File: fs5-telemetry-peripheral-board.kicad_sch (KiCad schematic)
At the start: 36 parts, among them J1 ATS668LSM, J2 Potentiometer, J3 Conn_01x10_Pin, J4 Strain Gauge, J5 1x8 Tire Surface Temperature 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, J6 Tire Temperature Sensor, J7 1x1 Tire Air Temperature Sens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, J8 Conn_01x09_Pin, J9 Conn_01x04_MountingPin, U1 LM2907M/NOPB, U2 LM7805CV, U3 INA125U, U4 ISO1050DUB

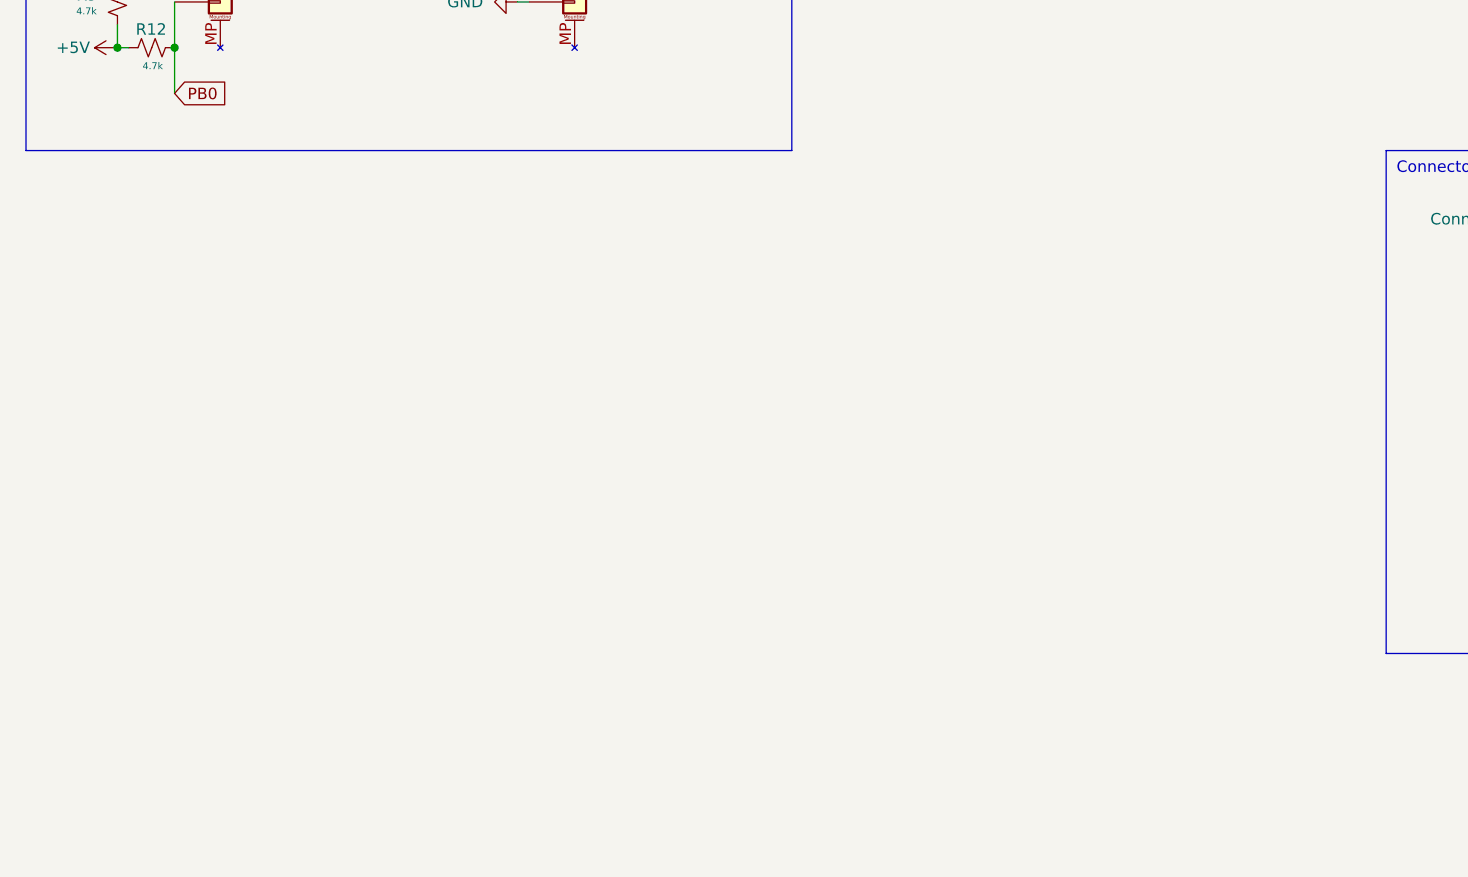
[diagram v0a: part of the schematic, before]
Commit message: added
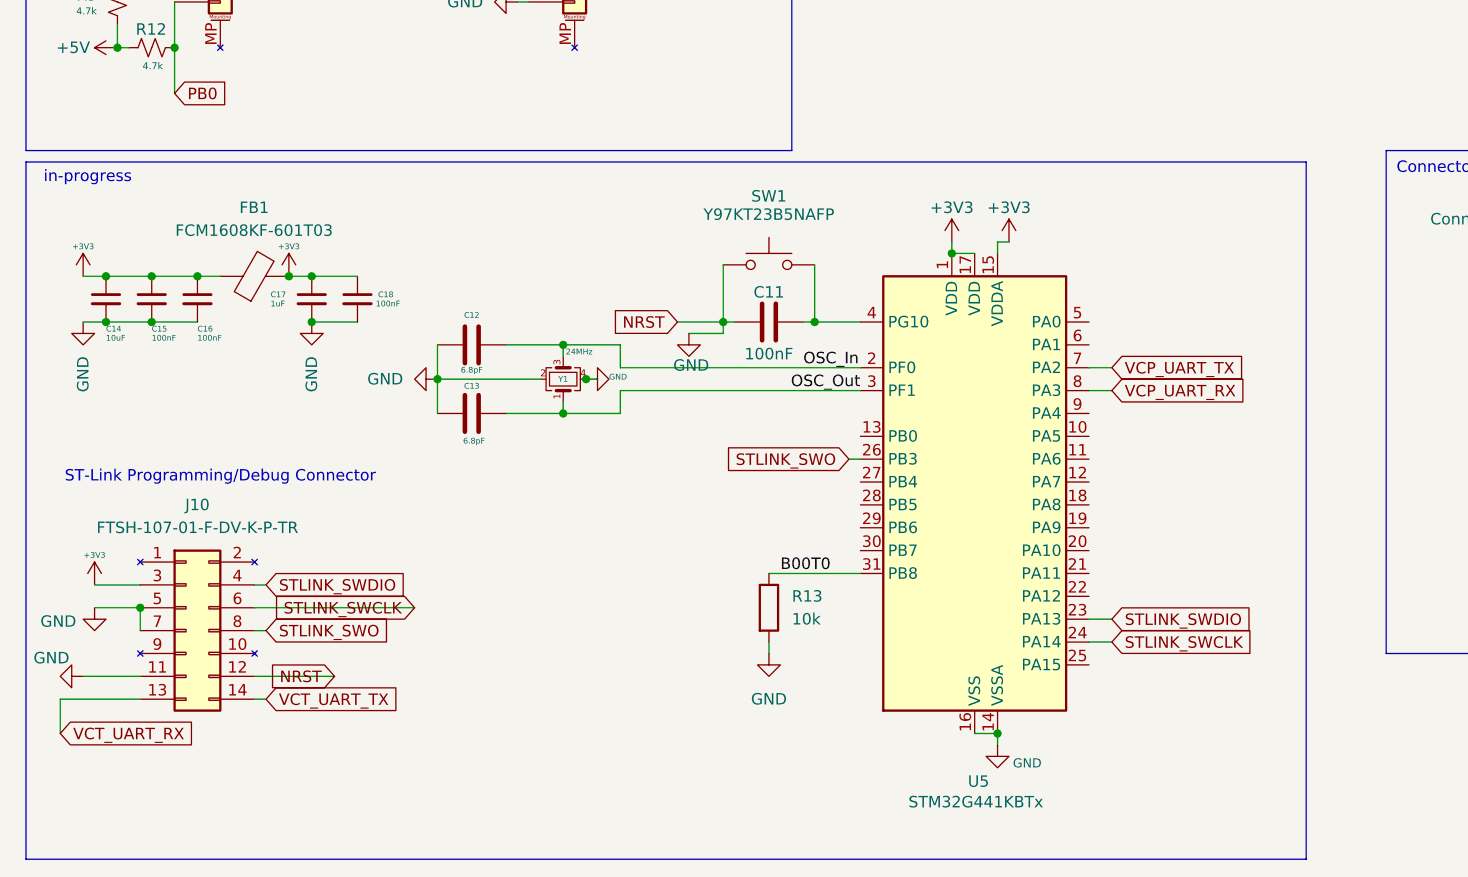
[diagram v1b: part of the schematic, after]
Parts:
- added C11: 100nF, symbol Device:C
- added C12, C13: 6.8pF, symbol Device:C
- added C14: 10uF, symbol Device:C_Small
- added C15, C16, C18: 100nF, symbol Device:C_Small
- added C17: 1uF, symbol Device:C_Small
- added FB1: FCM1608KF-601T03, symbol Device:FerriteBead
- added J10: FTSH-107-01-F-DV-K-P-TR, symbol Connector_Generic:Conn_02x07_Odd_Even
- added R13: 10k, symbol Device:R
- added SW1: Y97KT23B5NAFP, symbol Switch:SW_Push
- added U5: STM32G441KBTx, Package_QFP:LQFP-32_7x7mm_P0.8mm, symbol MCU_ST_STM32G4:STM32G441KBTx
- added Y1: 24MHz, symbol Device:Crystal_GND24_Small
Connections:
- net GND: now also C11.1, C12.1, C13.1, C14.2, C15.2, C16.2, C17.2, C18.2, J10.11 (Pin_11), J10.12 (Pin_12), J10.5 (Pin_5), J10.7 (Pin_7), R13.2, SW1.1, U5.14 (VSSA), U5.16 (VSS), U5.32 (VSS), Y1.2 (G), Y1.4 (G)
- new net: C11.2, SW1.2, U5.4 (PG10)
- new net +3V3: C14.1, C15.1, C16.1, C17.1, C18.1, FB1.1, FB1.2, J10.3 (Pin_3), U5.1 (VDD), U5.15 (VDDA), U5.17 (VDD)
- new net B00T0: R13.1, U5.31 (PB8)
- new net OSC_In: C12.2, U5.2 (PF0), Y1.3
- new net OSC_Out: C13.2, U5.3 (PF1), Y1.1
- new net STLINK_SWCLK: J10.6 (Pin_6), U5.24 (PA14)
- new net STLINK_SWDIO: J10.4 (Pin_4), U5.23 (PA13)
- new net STLINK_SWO: J10.8 (Pin_8), U5.26 (PB3)
- new net VCP_UART_RX: U5.8 (PA3)
- new net VCP_UART_TX: U5.7 (PA2)
- new net VCT_UART_RX: J10.13 (Pin_13)
- new net VCT_UART_TX: J10.14 (Pin_14)
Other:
- note added: "ST-Link Programming/Debug Connector"
- note added: "in-progress"
